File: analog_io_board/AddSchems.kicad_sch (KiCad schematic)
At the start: 11 parts, among them J2 DG245-5.0-02P, J3 DG245-5.0-02P, J4 DG245-5.0-02P, U5 L78L33 (SOT89)

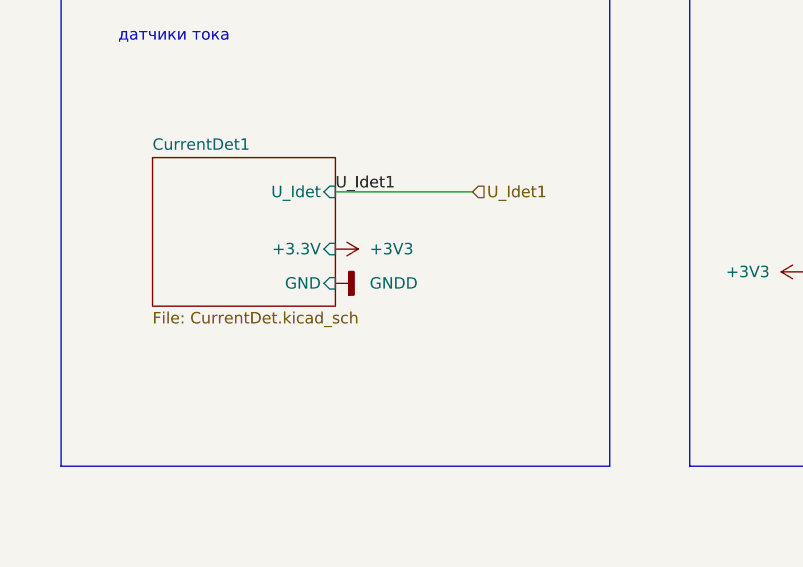
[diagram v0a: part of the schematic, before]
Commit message: analog board refresh pcb
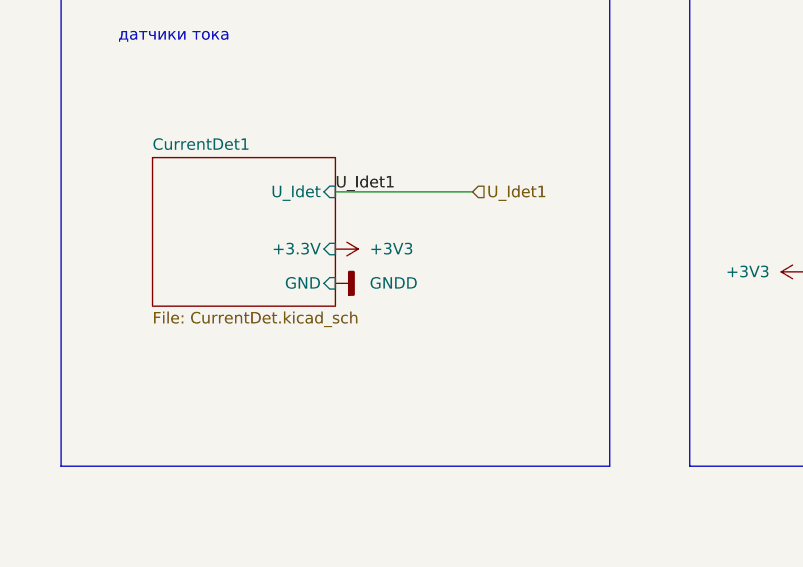
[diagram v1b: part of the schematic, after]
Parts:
- C18, C19: footprint Capacitor_SMD:C_0603_1608Metric_Pad1.08x0.95mm_HandSolder -> Capacitor_SMD:C_0603_1608Metric
- R9: footprint PCM_Resistor_SMD_AKL:R_1206_3216Metric_Pad1.42x1.75mm_HandSolder -> Resistor_SMD:R_1206_3216Metric
- TP16: footprint PCM_4ms_TestPoint:TestPoint_D1 -> TestPoint:TestPoint_Pad_D1.0mm
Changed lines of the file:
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@@
 	)
 	(symbol
-		(lib_id "PCM_4ms_Power-symbol:GNDA")
+		(lib_id "power:GNDA")
 		(at 86.36 186.69 0)
 		(unit 1)
@@
 			)
 		)
-		(property "Description" ""
+		(property "Description" "Power symbol creates a global label with name \"GNDA\" , analog ground"
 			(at 86.36 186.69 0)
 			(effects
@@
 	)
 	(symbol
-		(lib_id "PCM_4ms_Power-symbol:GNDA")
+		(lib_id "power:GNDA")
 		(at 31.75 181.61 0)
 		(unit 1)
@@
 			)
 		)
-		(property "Description" ""
+		(property "Description" "Power symbol creates a global label with name \"GNDA\" , analog ground"
 			(at 31.75 181.61 0)
 			(effects
@@
 			)
 		)
-		(property "Description" ""
+		(property "Description" "Generic connector, single row, 01x02, script generated (kicad-library-utils/schlib/autogen/connector/)"
 			(at 257.81 101.6 0)
 			(effects
@@
 	)
 	(symbol
-		(lib_id "PCM_4ms_Power-symbol:GNDA")
+		(lib_id "power:GNDA")
 		(at 63.5 186.69 0)
 		(unit 1)
@@
 			)
 		)
-		(property "Description" ""
+		(property "Description" "Power symbol creates a global label with name \"GNDA\" , analog ground"
 			(at 63.5 186.69 0)
 			(effects
@@
 			)
 		)
-		(property "Description" ""
+		(property "Description" "Voltage dependent resistor"
 			(at 218.44 102.87 0)
 			(effects
@@
 			)
 		)
-		(property "Sim.Library" "${KICAD7_SYMBOL_DIR}/Simulation_SPICE.sp"
+		(property "Sim.Library" "${KICAD9_SYMBOL_DIR}/Simulation_SPICE.sp"
 			(at 218.44 102.87 0)
 			(effects
@@
 			)
 		)
-		(property "Description" ""
+		(property "Description" "Power symbol creates a global label with name \"+24V\""
 			(at 135.89 50.8 0)
 			(effects
@@
 			)
 		)
-		(property "Description" ""
+		(property "Description" "Power symbol creates a global label with name \"+3V3\""
 			(at 195.58 129.54 0)
 			(effects
@@
 			)
 		)
-		(property "Description" ""
+		(property "Description" "Fuse"
 			(at 241.3 104.14 0)
 			(effects
@@
 			)
 		)
-		(property "Description" ""
+		(property "Description" "Power symbol creates a global label with name \"+3V3\""
 			(at 52.07 48.26 0)
 			(effects
@@
 			)
 		)
-		(property "Footprint" "PCM_4ms_TestPoint:TestPoint_D1"
+		(property "Footprint" "TestPoint:TestPoint_Pad_D1.0mm"
 			(at 93.98 177.8 0)
 			(effects
@@
 			)
 		)
-		(property "Description" ""
+		(property "Description" "test point"
 			(at 93.98 172.72 0)
 			(effects
@@
 		)
 		(property "Value" "GNDD"
-			(at 55.88 52.07 90)
+			(at 55.88 52.0699 90)
 			(effects
 				(font
@@
 			)
 		)
-		(property "Description" ""
+		(property "Description" "Power symbol creates a global label with name \"GNDD\" , digital ground"
 			(at 52.07 52.07 0)
 			(effects
@@
 			)
 		)
-		(property "Description" ""
+		(property "Description" "Power symbol creates a global label with name \"+3V3\""
 			(at 35.56 144.78 0)
 			(effects
@@
 			)
 		)
-		(property "Footprint" "PCM_Resistor_SMD_AKL:R_1206_3216Metric_Pad1.42x1.75mm_HandSolder"
+		(property "Footprint" "Resistor_SMD:R_1206_3216Metric"
 			(at 52.07 170.942 90)
 			(effects
@@
 			)
 		)
-		(property "Description" ""
+		(property "Description" "Resistor"
 			(at 52.07 172.72 0)
 			(effects
@@
 			)
 		)
-		(property "Footprint" "Capacitor_SMD:C_0603_1608Metric_Pad1.08x0.95mm_HandSolder"
+		(property "Footprint" "Capacitor_SMD:C_0603_1608Metric"
 			(at 64.4652 186.69 0)
 			(effects
@@
 			)
 		)
-		(property "Description" ""
+		(property "Description" "Unpolarized capacitor"
 			(at 63.5 182.88 0)
 			(effects
@@
 			)
 		)
-		(property "Description" ""
+		(property "Description" "Power symbol creates a global label with name \"+3V3\""
 			(at 104.14 50.8 0)
 			(effects
@@
 			)
 		)
-		(property "Description" ""
+		(property "Description" "Generic connector, single row, 01x02, script generated (kicad-library-utils/schlib/autogen/connector/)"
 			(at 255.27 137.16 0)
 			(effects
@@
 			)
 		)
-		(property "Description" ""
+		(property "Description" "Power symbol creates a global label with name \"+24V\""
 			(at 35.56 170.18 0)
 			(effects
@@
 			)
 		)
-		(property "Description" ""
+		(property "Description" "Generic connector, single row, 01x02, script generated (kicad-library-utils/schlib/autogen/connector/)"
 			(at 255.27 123.19 0)
 			(effects
@@
 			)
 		)
-		(property "Description" ""
+		(property "Description" "Power symbol creates a global label with name \"+3V3\""
 			(at 195.58 154.94 0)
 			(effects
@@
 			)
 		)
-		(property "Footprint" "Capacitor_SMD:C_0603_1608Metric_Pad1.08x0.95mm_HandSolder"
+		(property "Footprint" "Capacitor_SMD:C_0603_1608Metric"
 			(at 87.3252 186.69 0)
 			(effects
@@
 			)
 		)
-		(property "Description" ""
+		(property "Description" "Unpolarized capacitor"
 			(at 86.36 182.88 0)
 			(effects
@@
 			)
 		)
-		(property "Description" ""
+		(property "Description" "Power symbol creates a global label with name \"+3.3VA\""
 			(at 93.98 167.64 0)
 			(effects
@@
 			)
 		)
-		(property "Description" ""
+		(property "Description" "Fuse"
 			(at 241.3 101.6 0)
 			(effects
@@
 	)
 	(symbol
-		(lib_id "PCM_4ms_Power-symbol:GNDA")
+		(lib_id "power:GNDA")
 		(at 77.47 180.34 0)
 		(unit 1)
@@
 			)
 		)
-		(property "Description" ""
+		(property "Description" "Power symbol creates a global label with name \"GNDA\" , analog ground"
 			(at 77.47 180.34 0)
 			(effects
@@
 	)
 	(symbol
-		(lib_id "PCM_4ms_Power-symbol:GNDA")
+		(lib_id "power:GNDA")
 		(at 134.62 60.96 0)
 		(unit 1)
@@
 			)
 		)
-		(property "Description" ""
+		(property "Description" "Power symbol creates a global label with name \"GNDA\" , analog ground"
 			(at 134.62 60.96 0)
 			(effects
@@
 			)
 		)
-		(property "Description" ""
+		(property "Description" "Power symbol creates a global label with name \"+3V3\""
 			(at 179.07 105.41 0)
 			(effects
@@
 			)
 		)
-		(property "Description" ""
+		(property "Description" "Power symbol creates a global label with name \"GNDD\" , digital ground"
 			(at 35.56 152.4 0)
 			(effects
@@
 			)
 		)
-		(property "Description" ""
+		(property "Description" "Power symbol creates a global label with name \"+3.3VA\""
 			(at 35.56 137.16 0)
 			(effects
@@
 			)
 		)
-		(property "Description" ""
+		(property "Description" "Positive 100mA 30V Linear Regulator, Fixed Output 3.3V, SOT-89"
 			(at 77.47 172.72 0)
 			(effects
